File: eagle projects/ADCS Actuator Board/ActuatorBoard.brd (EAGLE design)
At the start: 91 x 91 mm, 278 parts, among them J19 TE_1-84953-1, J20 TE_1-84953-1, J21 TE_1-84953-1, U10 DRV10970_MOTOR_DRIVERDRV10970, U12 DRV10970_MOTOR_DRIVERDRV10970, U13 ADS7841E_2K5, U15 TLV9051IDCKR, U19 TLV9051IDCKR, U2 ADS7841E_2K5, U21 TLV9051IDCKR, U23 TLV9051IDCKR, U24 TLV9051IDCKR, U25 ADS7841E_2K5, U26 TLV9051IDCKR, U27 ADS7841E_2K5, U28 TLV9051IDCKR, U29 TLV9051IDCKR, U3 ADS7841E_2K5, U30 TLV9051IDCKR, U31 TLV9051IDCKR, U32 TLV9051IDCKR, U34 TVS991, U35 BD6210F-E2, U38 TVS991, U39 BD6210F-E2, U4 ADS7841E_2K5, U5 TVS991, U6 TLV9051IDCKR, U7 DRV10970_MOTOR_DRIVERDRV10970, U9 BD6210F-E2

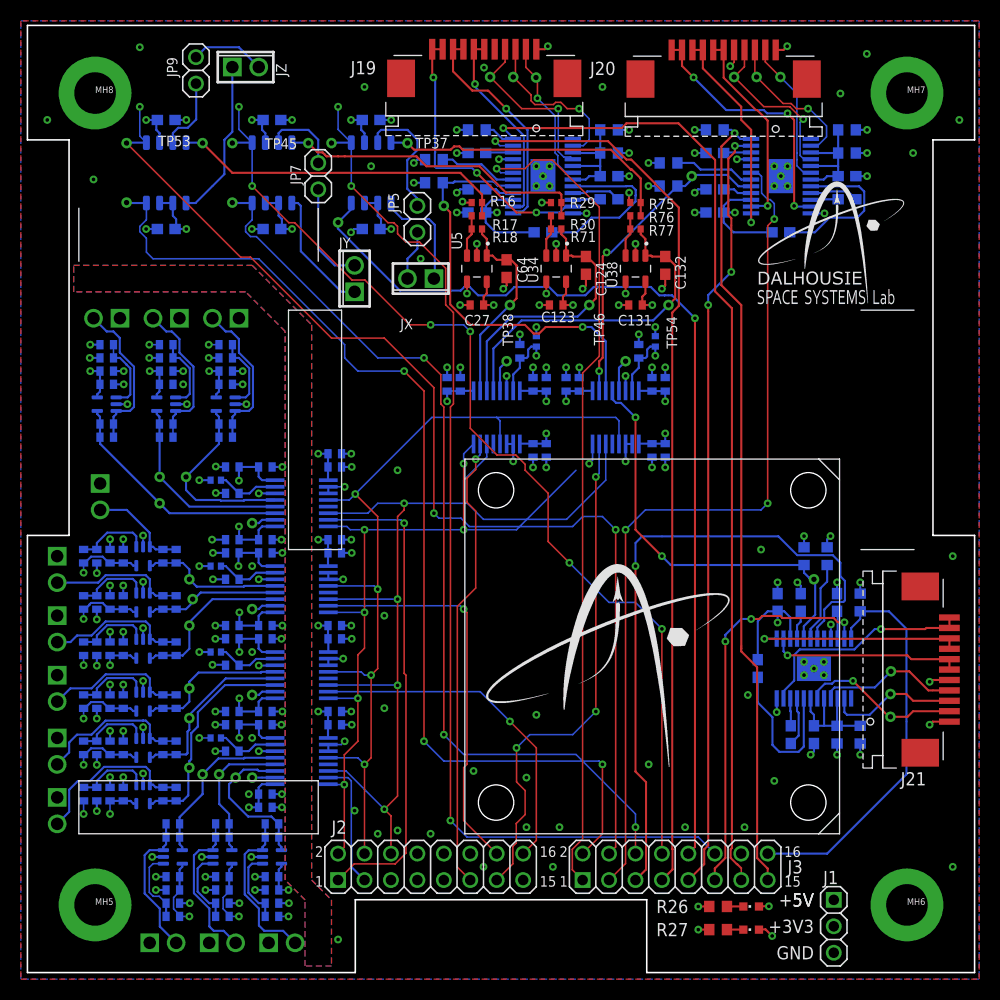
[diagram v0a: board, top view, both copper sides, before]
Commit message: solved drc errors
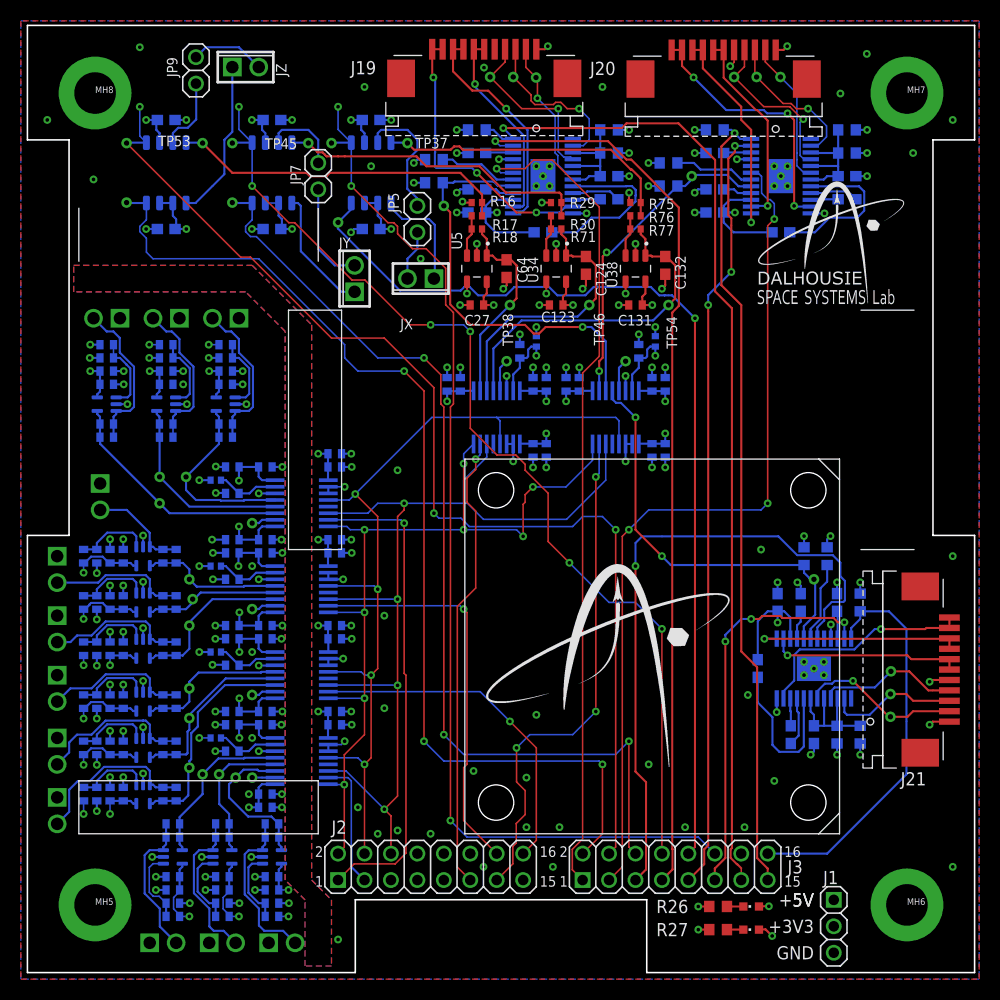
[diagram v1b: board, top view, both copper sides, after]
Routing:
- net UCB0_SPI_CLK: track 77.0 -> 81.9 mm, vias 7 -> 8
- net MAG_Y_FIN: track 89.5 -> 94.2 mm
